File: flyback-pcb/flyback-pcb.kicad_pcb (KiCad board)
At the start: 2 copper layers, 48 parts, among them Q3 MMBTA06, U1 MIN1072M-TL, U2 INN3865CH801TL

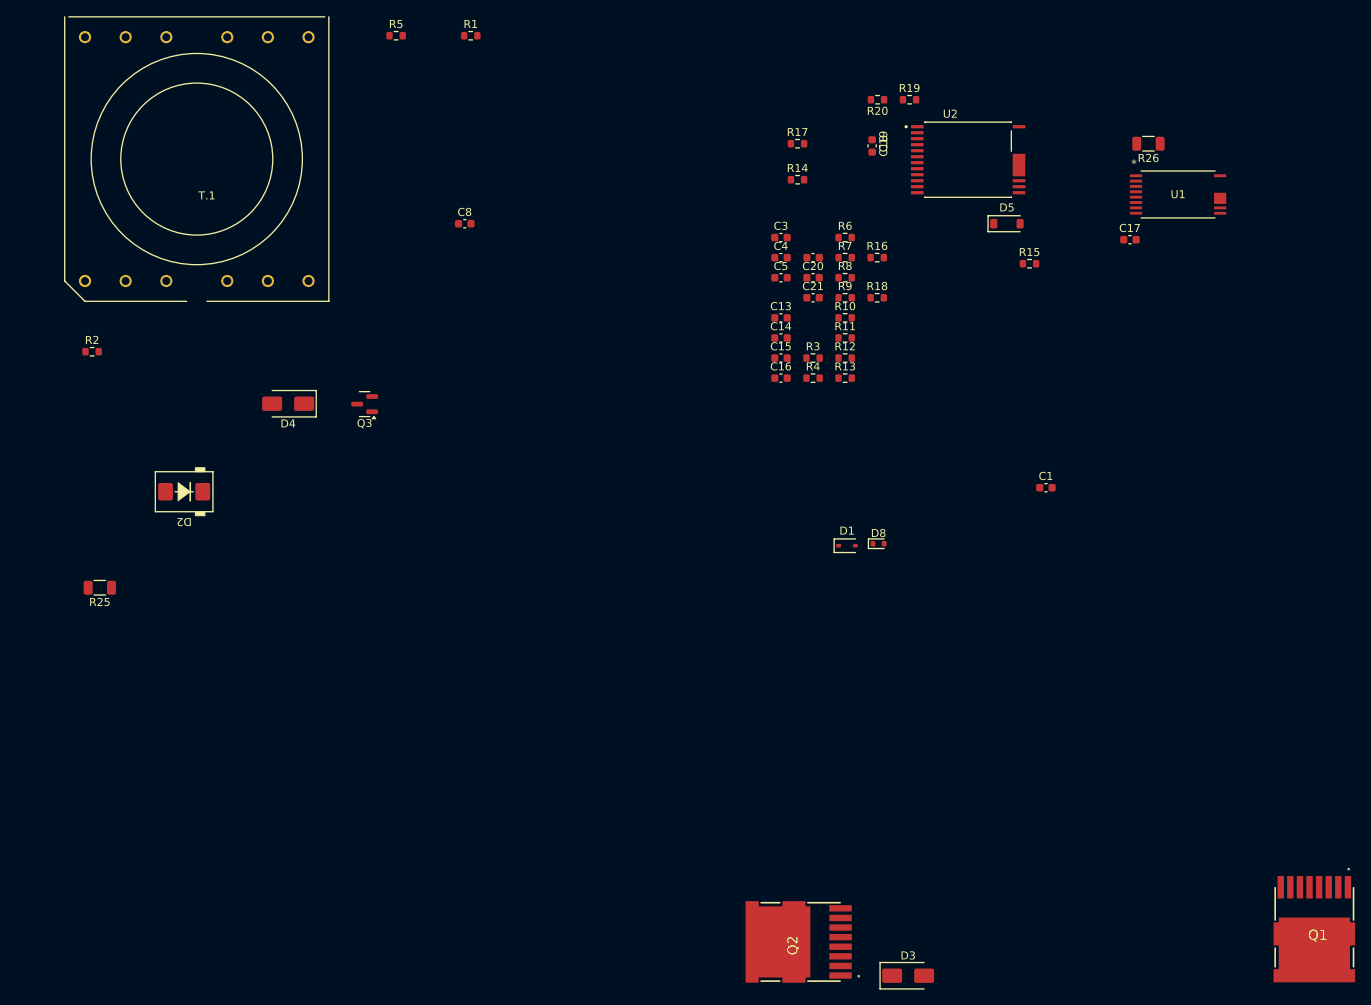
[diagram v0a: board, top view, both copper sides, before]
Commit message: Re_design
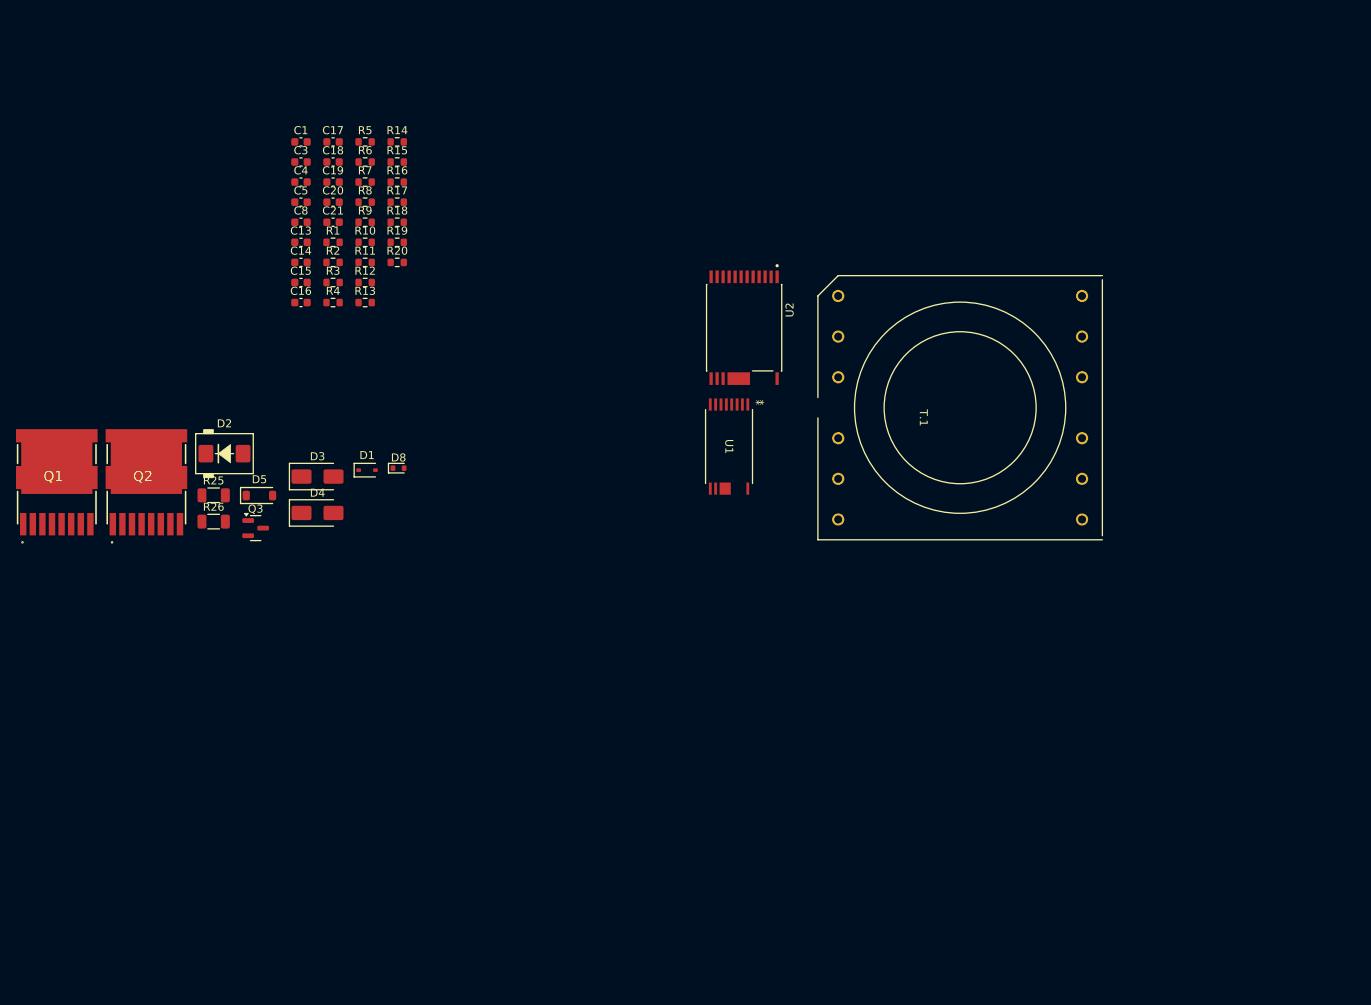
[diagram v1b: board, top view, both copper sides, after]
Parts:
- moved Q1 166.8 mm to (55.1, 92.8), turned to 0 degrees
- moved R26 126.0 mm to (74.7, 97.7), turned to 0 degrees
- moved C1 102.7 mm to (85.6, 50.3)
- moved C17 100.4 mm to (89.6, 50.3)
- moved Q2 99.7 mm to (66.3, 92.8), turned to 0 degrees
- moved D5 99.4 mm to (80.4, 94.5)
- moved D3 96.7 mm to (87.7, 92.1)
- moved T.1 93.2 mm to (162.9, 84.8), turned to -90 degrees
- moved R15 80.1 mm to (97.6, 52.8)
- moved C18 67.4 mm to (89.6, 52.8), turned to 0 degrees
- moved R19 66.5 mm to (97.6, 62.8)
- moved U1 64.4 mm to (139.1, 88.4), turned to -90 degrees
- moved R20 63.4 mm to (97.6, 65.3), turned to 0 degrees
- moved D1 60.7 mm to (93.9, 91.3)
- moved D8 60.7 mm to (97.8, 91.1)
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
